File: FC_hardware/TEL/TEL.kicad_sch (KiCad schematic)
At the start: 15 parts, among them J1 Conn_01x14, J2 Conn_01x01_Pin, U1 LIS3MDL, U2 Ai-Thinker-Ra-02, U3 TESEO-LIV4F

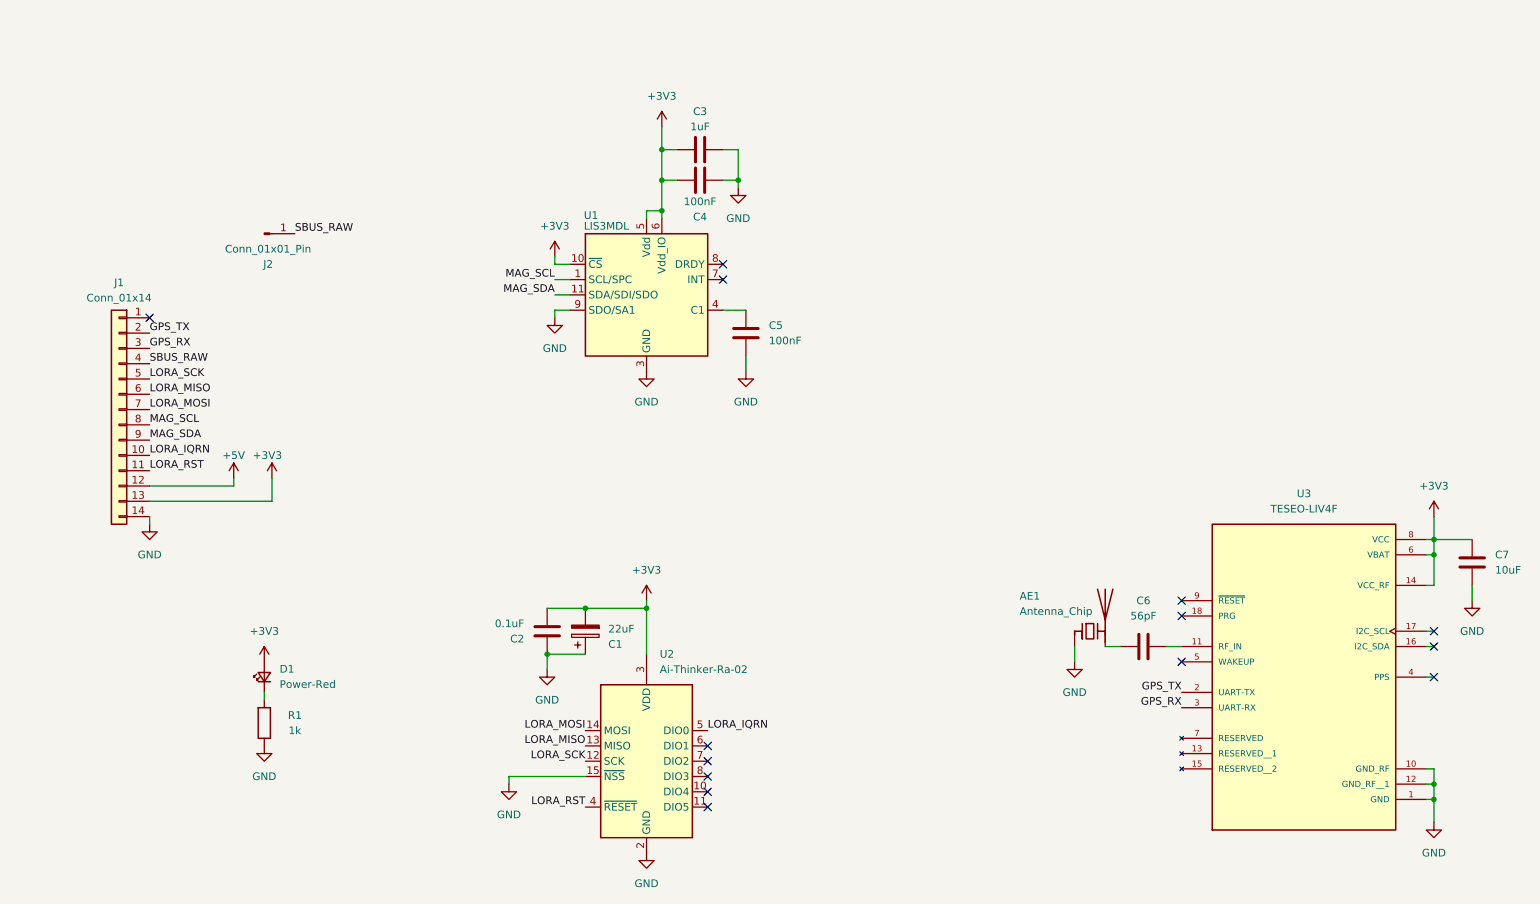
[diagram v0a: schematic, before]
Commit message: Clean up
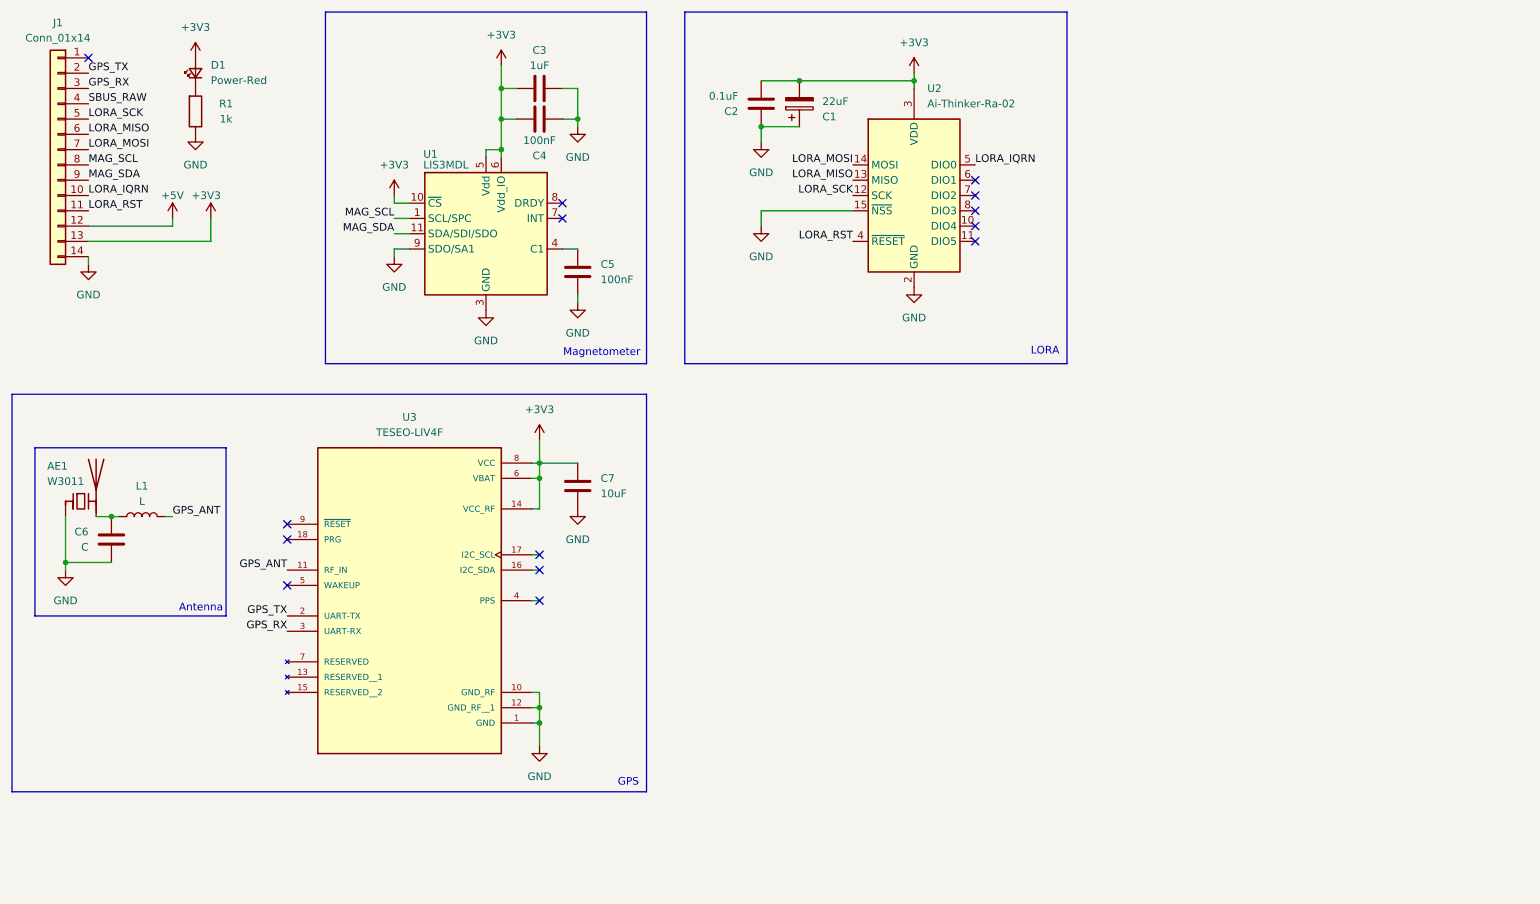
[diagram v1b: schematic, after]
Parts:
- removed J2: Conn_01x01_Pin, Connector_PinHeader_1.27mm:PinHeader_1x01_P1.27mm_Vertical, symbol Connector:Conn_01x01_Pin
- added L1: L, symbol Device:L
- AE1: value Antenna_Chip -> W3011
- C6: value 56pF -> C
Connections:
- net GND: now also C6.2
- net at AE1.2 (PCB_Trace): now also C6.1, L1.1; no longer C6.2
- net GPS_ANT: now reaches U3.11 (RF_IN)
- net GPS_ANT: now also L1.2; no longer C6.1
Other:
- note added: "Antenna"
- note added: "GPS"
- note added: "LORA"
- note added: "Magnetometer"
- moved on the sheet: AE1, C1, C2, C3, C4, C5, C6, C7, D1, J1, R1, U1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
